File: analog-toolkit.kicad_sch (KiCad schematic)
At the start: 53 parts, among them J1 USB_C, J2 IO, J3 UART, J4 I2C, J5 VBUS, J6 3.3V, J7 OPAMP, J8 ADC, P1 TC2030, Q1 AO3400A, SW1 DFU, U1 AP2204R-3.3, U2 otter_USBLC6-4, U3 STM32G431xB

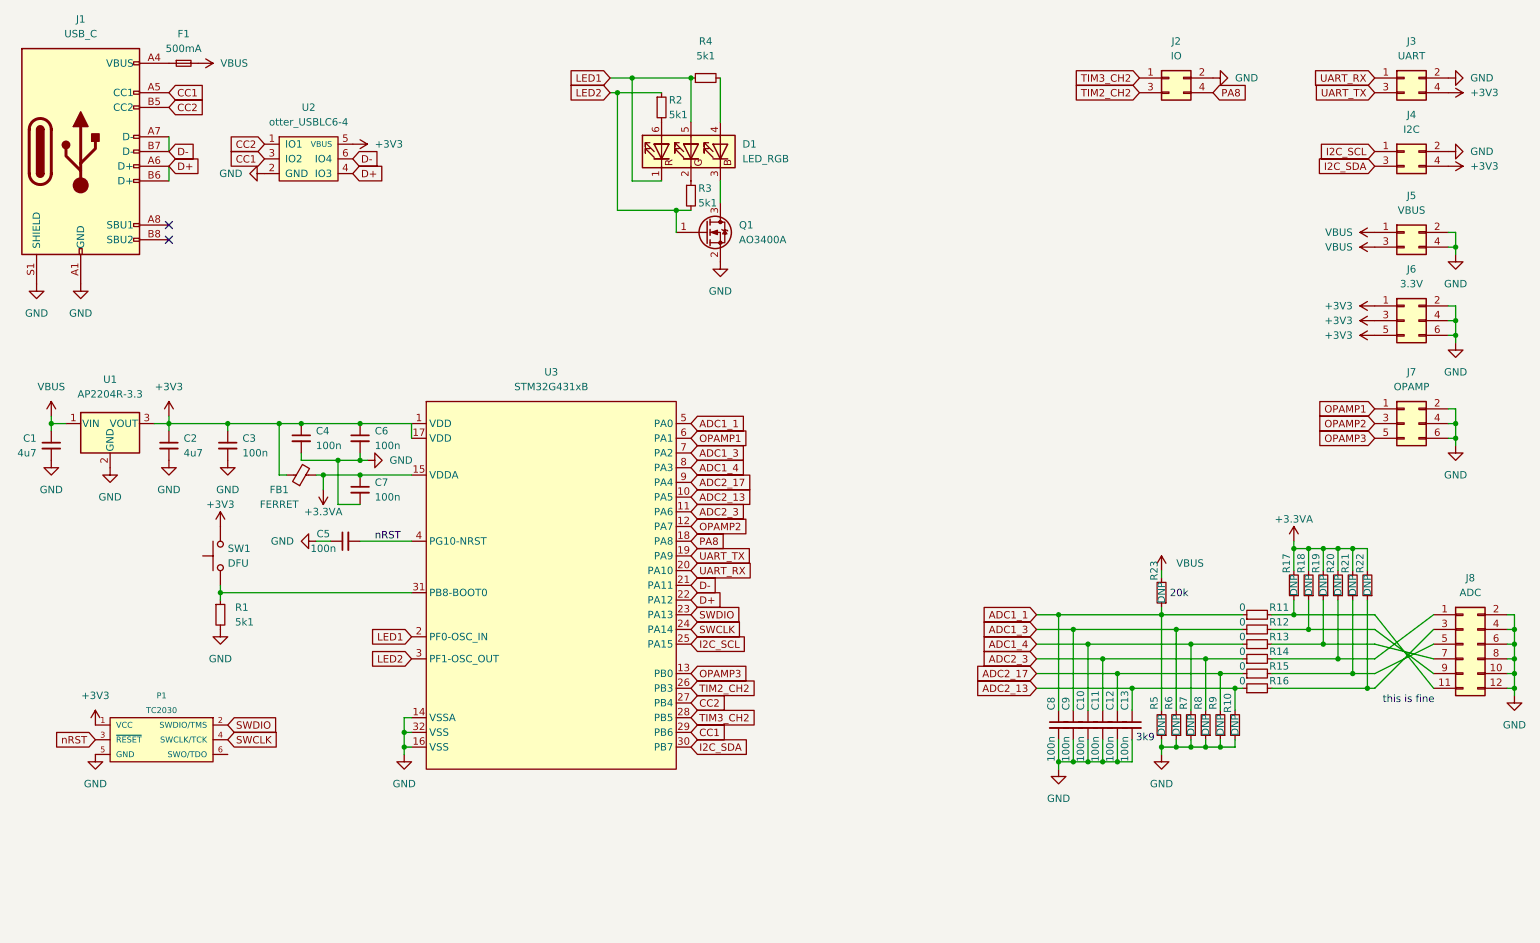
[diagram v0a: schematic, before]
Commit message: updated version
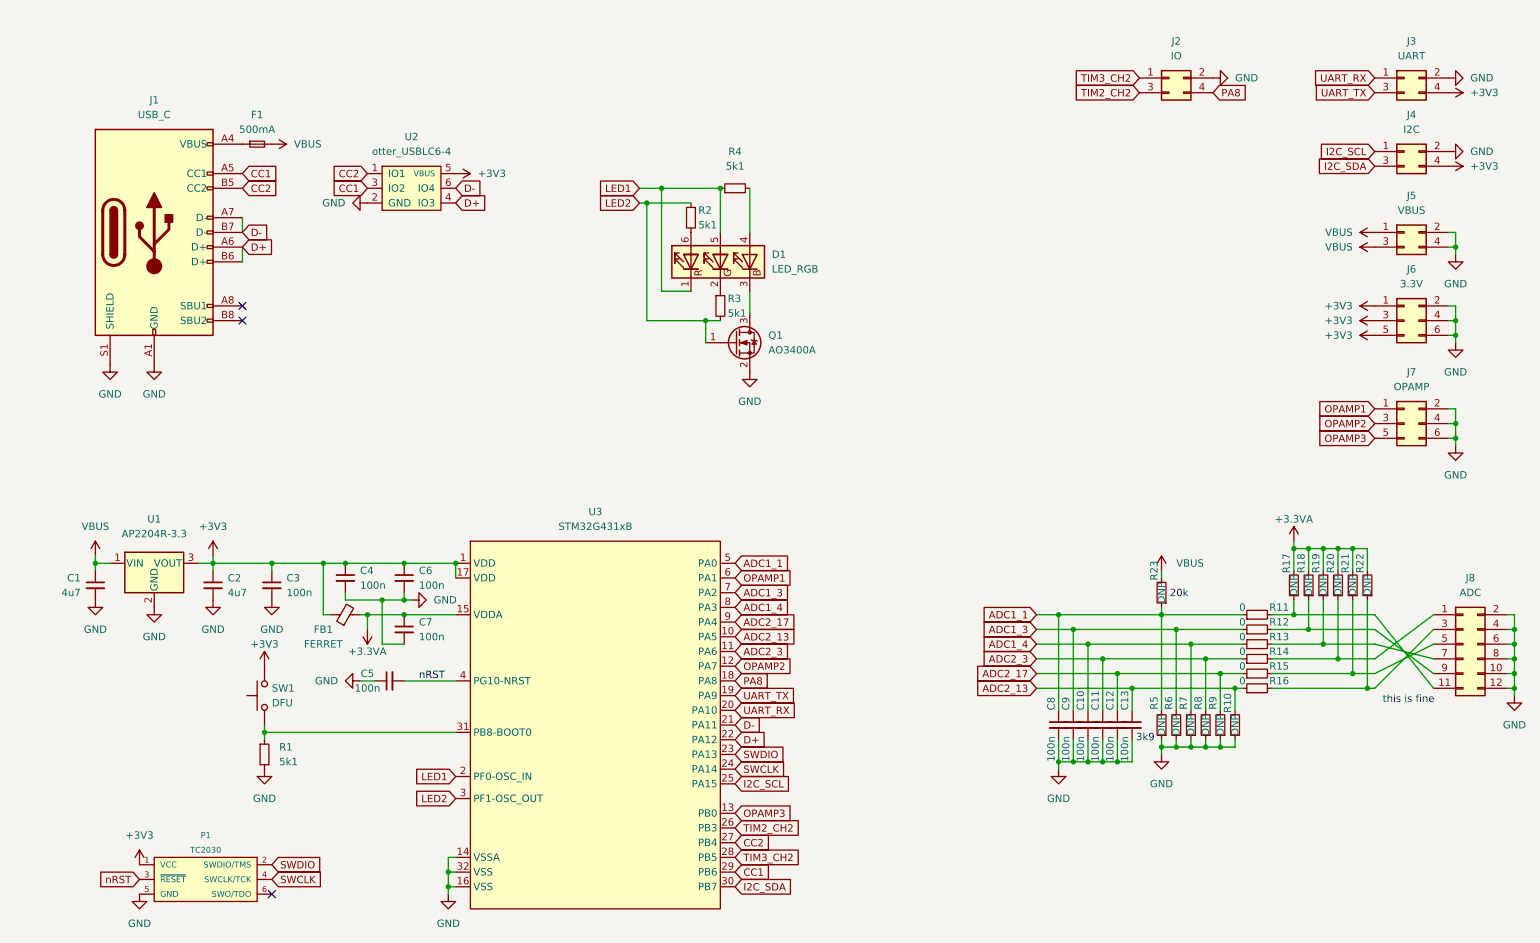
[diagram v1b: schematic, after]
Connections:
- no-connect marks 2 -> 3
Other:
- moved on the sheet: C1, C2, C3, C4, C5, C6, C7, D1, F1, FB1, J1, P1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
